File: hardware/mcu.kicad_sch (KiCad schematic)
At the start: 2 parts, among them J3 Conn_ARM_SWD_TagConnect_TC203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, U1 nRF52832-QFxx

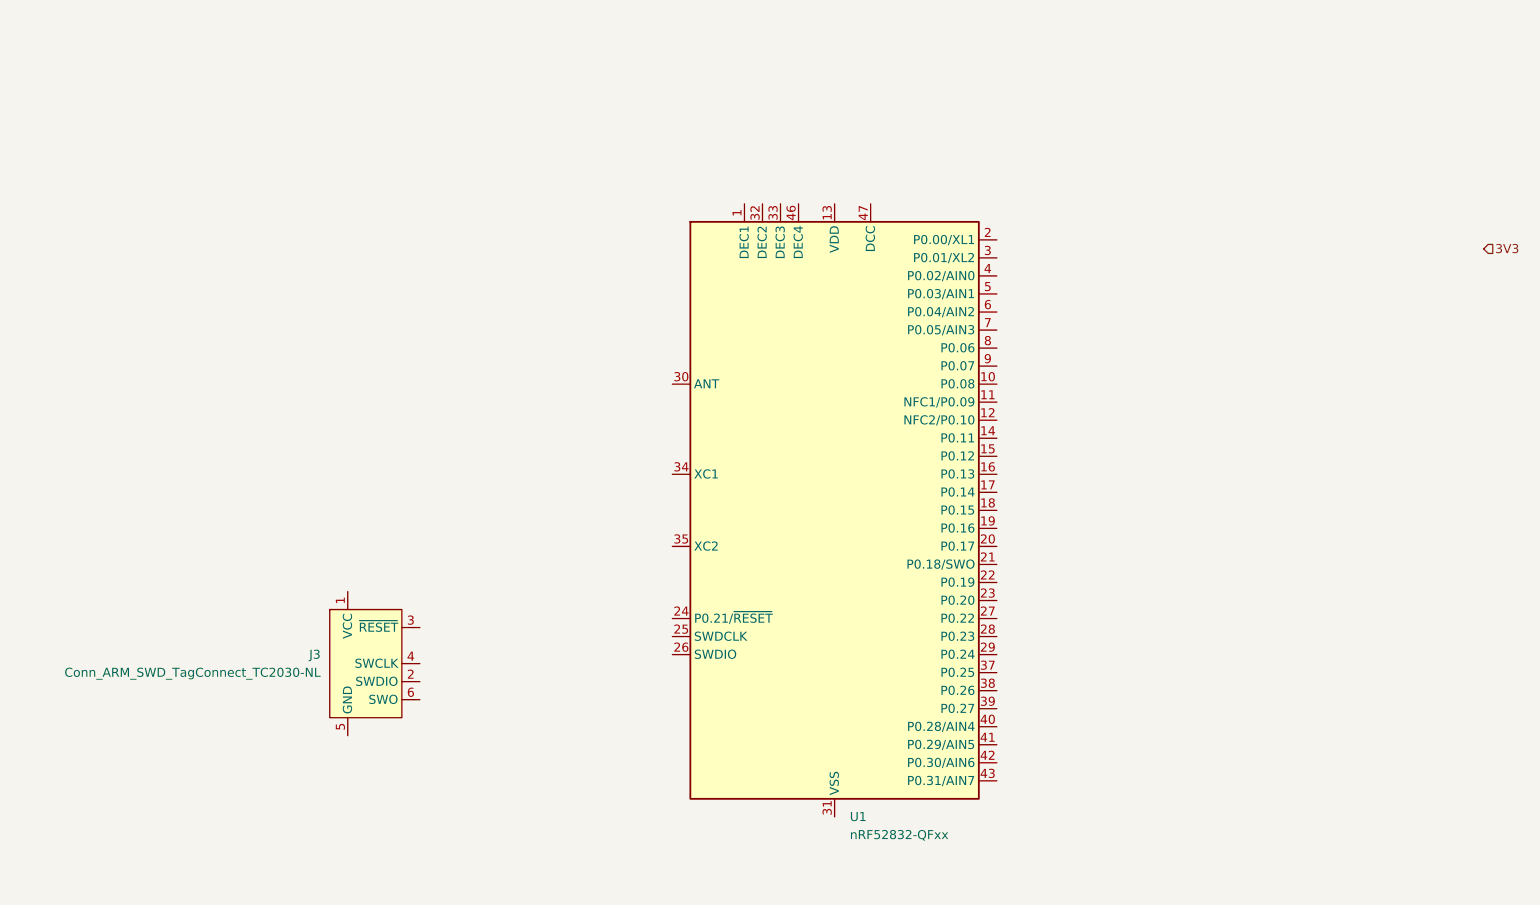
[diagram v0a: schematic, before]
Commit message: finished first draft of schematic, need to review
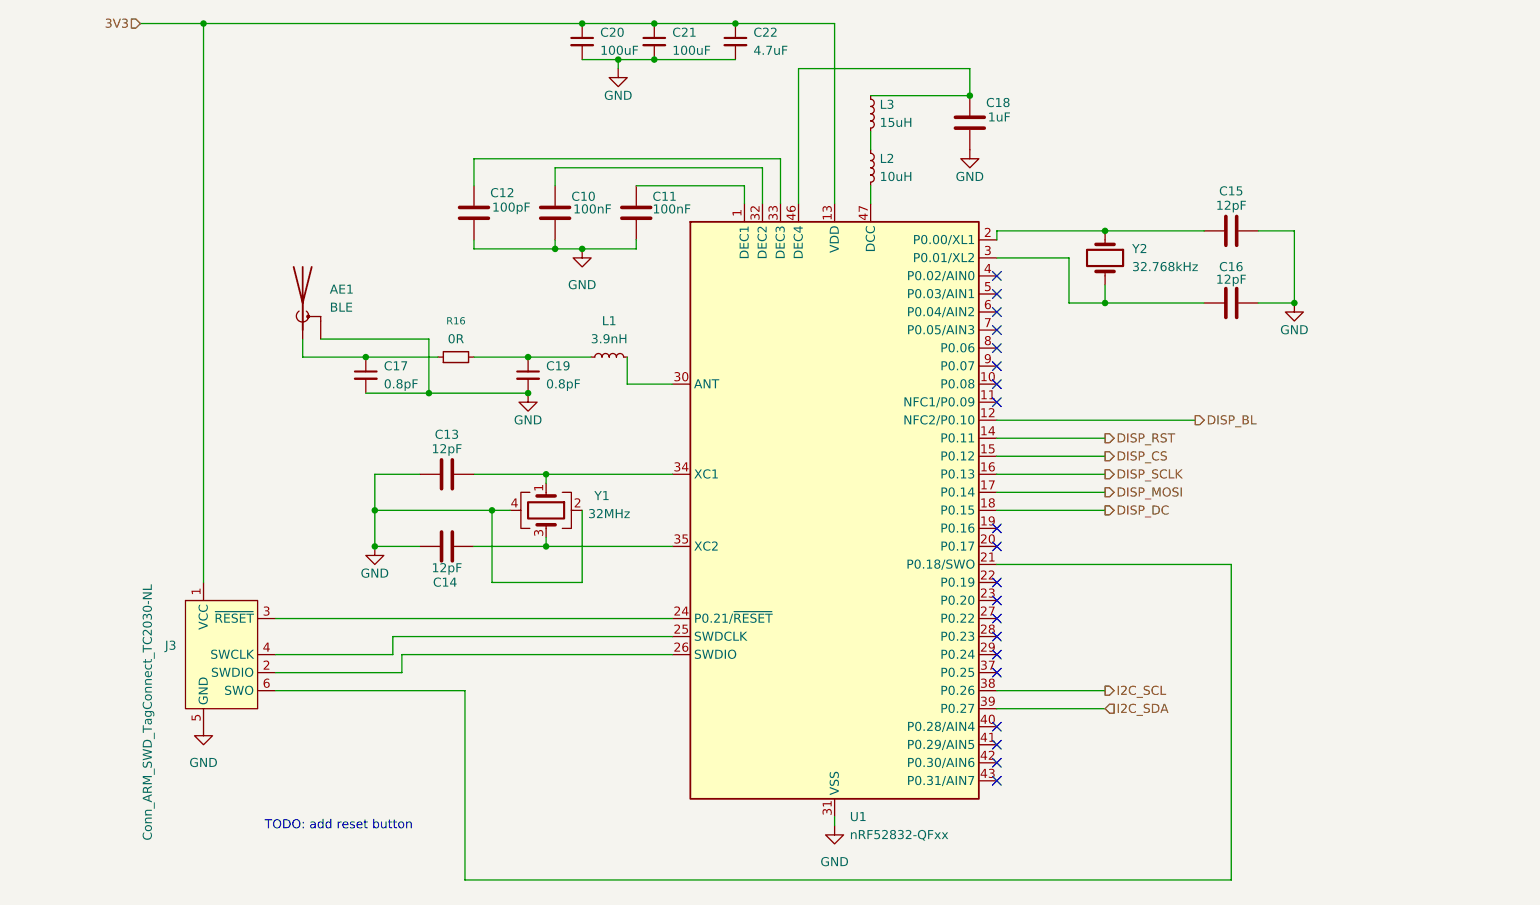
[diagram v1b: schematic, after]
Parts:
- added AE1: BLE, symbol Device:Antenna_Shield
- added C10, C11: 100nF, symbol Device:C
- added C12: 100pF, symbol Device:C
- added C13, C14, C15, C16: 12pF, symbol Device:C
- added C17, C19: 0.8pF, symbol Device:C_Small
- added C18: 1uF, symbol Device:C
- added C20, C21: 100uF, symbol Device:C_Small
- added C22: 4.7uF, symbol Device:C_Small
- added L1: 3.9nH, symbol Device:L_Small
- added L2: 10uH, symbol Device:L_Small
- added L3: 15uH, symbol Device:L_Small
- added R16: 0R, symbol Device:R_Small
- added Y1: 32MHz, symbol Device:Crystal_GND24
- added Y2: 32.768kHz, symbol Device:Crystal
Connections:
- net 3V3: now also J3.1 (VCC), U1.13 (VDD), U1.36 (VDD), U1.48 (VDD), C20.1, C21.1, C22.1
- net at U1.1 (DEC1): now also C11.1
- net DISP_BL: now reaches U1.12 (NFC2/P0.10)
- net DISP_RST: now reaches U1.14 (P0.11)
- net DISP_CS: now reaches U1.15 (P0.12)
- net DISP_SCLK: now reaches U1.16 (P0.13)
- net DISP_MOSI: now reaches U1.17 (P0.14)
- net DISP_DC: now reaches U1.18 (P0.15)
- net at U1.2 (P0.00/XL1): now also C15.1, Y2.1
- net at U1.21 (P0.18/SWO): now also J3.6 (SWO)
- net at U1.24 (P0.21/~{RESET}): now also J3.3 (~{RESET})
- net at U1.25 (SWDCLK): now also J3.4 (SWCLK)
- net at U1.26 (SWDIO): now also J3.2 (SWDIO)
- net at U1.3 (P0.01/XL2): now also C16.1, Y2.2
- net at U1.30 (ANT): now also L1.2
- net GND: now reaches U1.31 (VSS), U1.45 (VSS), U1.49 (VSS)
- net GND: now also J3.5 (GND), AE1.2 (Shield), C10.1, C11.2, C12.2, C13.1, C14.1, C15.2, C16.2, C17.2, C18.2, C19.2, C20.2, C21.2, C22.2, Y1.2, Y1.4
- net at U1.32 (DEC2): now also C10.2
- net at U1.33 (DEC3): now also C12.1
- net at U1.34 (XC1): now also C13.2, Y1.1
- net at U1.35 (XC2): now also C14.2, Y1.3
- net I2C_SCL: now reaches U1.38 (P0.26)
- net I2C_SDA: now reaches U1.39 (P0.27)
- net at U1.46 (DEC4): now also C18.1, L3.1
- net at U1.47 (DCC): now also L2.2
- new net: AE1.1 (A), C17.1, R16.1
- new net: C19.1, L1.1, R16.2
- new net: L2.1, L3.2
- no-connect marks 0 -> 20
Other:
- note added: "TODO: add reset button"
- moved on the sheet: J3
